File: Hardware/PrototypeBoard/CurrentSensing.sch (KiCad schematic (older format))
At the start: 6 parts, among them U1 TLI4970-D025T4, U2 TLI4970-D025T4, U3 TLI4970-D025T4

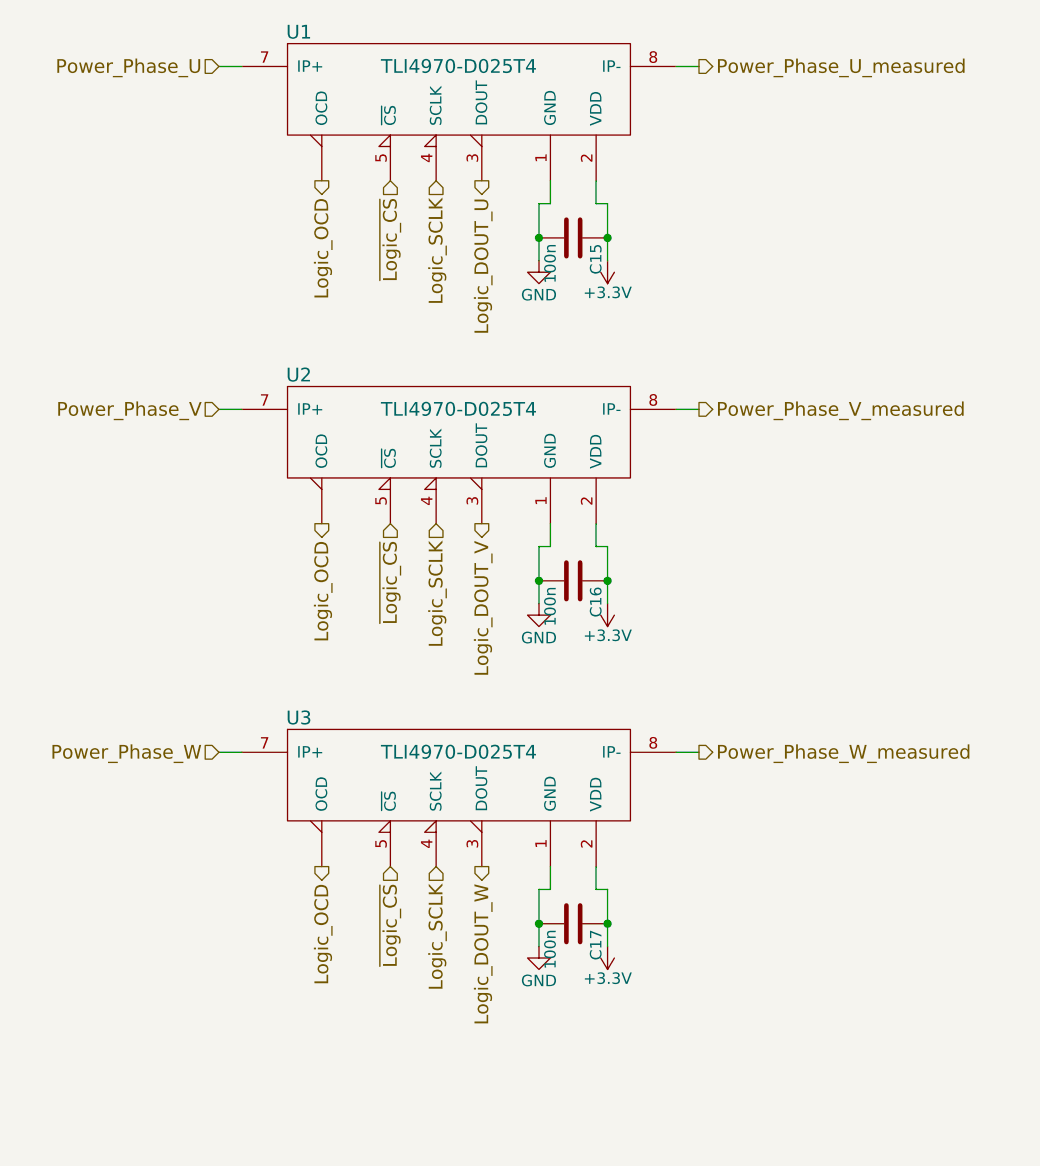
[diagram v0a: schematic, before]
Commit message: some more layout...
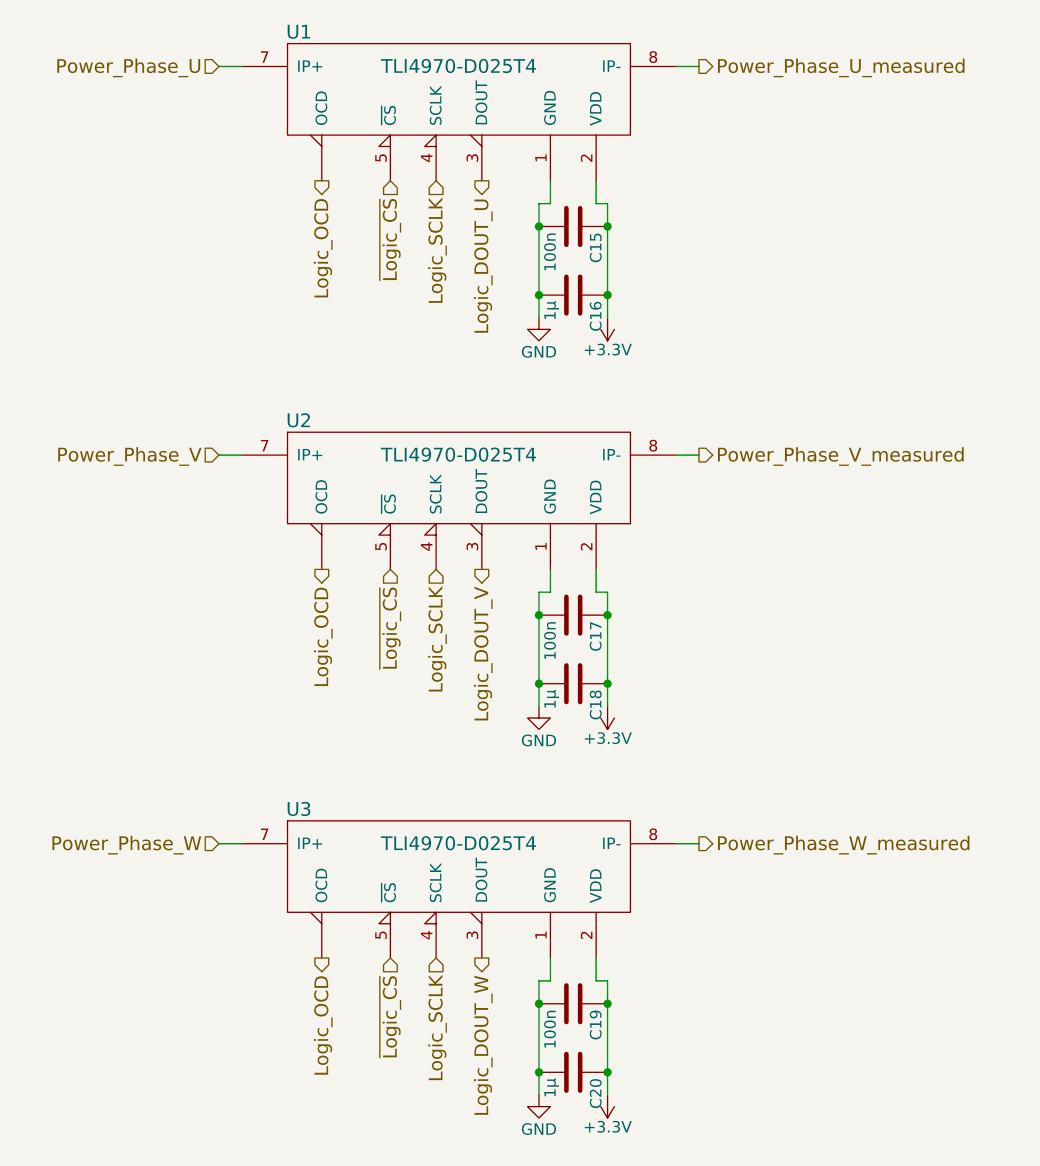
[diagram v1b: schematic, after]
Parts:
- removed C17: 100n, Capacitors_SMD:C_0805_HandSoldering, symbol C
- added C15, C19: 100n, Capacitors_SMD:C_0805_HandSoldering, symbol C
- added C18, C20: 1μ, Capacitors_SMD:C_0805_HandSoldering, symbol C
- C16: value 100n -> 1μ
- renumbered C15 to C17
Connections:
- net +3V3: now also C15.1, C18.1, C19.1, C20.1
- net GND: now also C15.2, C18.2, C19.2, C20.2
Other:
- moved on the sheet: C17, U2, U3
